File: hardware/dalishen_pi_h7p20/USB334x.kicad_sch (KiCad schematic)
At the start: 21 parts, among them J2 USB_C_Receptacle_USB2.0_16P, J3 USB_A, SW6 SW_DPDT_x2, U20 USB3343, Y1 26M

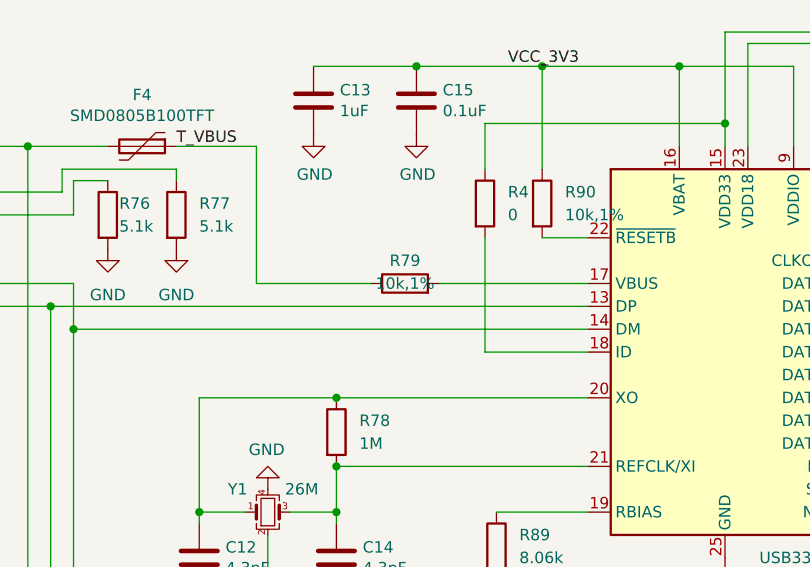
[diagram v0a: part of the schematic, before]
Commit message: [dalishen_pi_h7p20] 待review
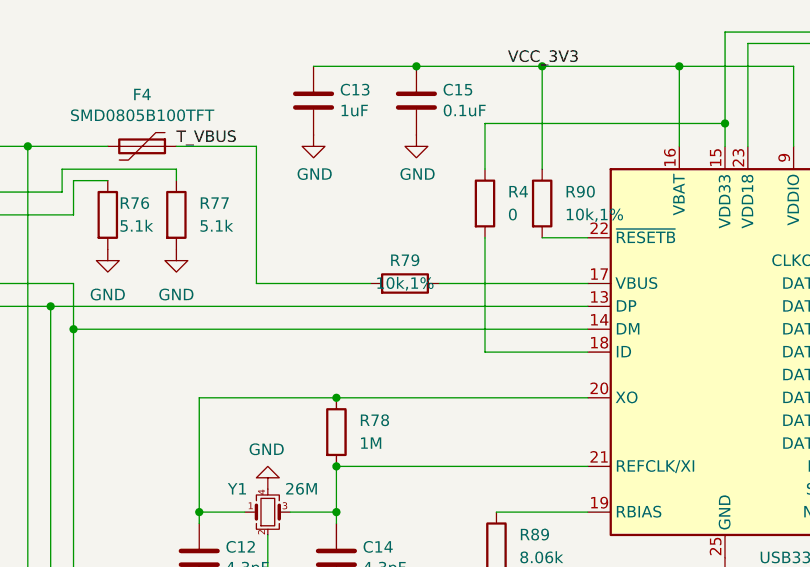
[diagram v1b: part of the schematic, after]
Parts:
- SW6: footprint Button_Switch_SMD:SW_DIP_SPSTx03_Slide_KingTek_DSHP03TJ_W5.25mm_P1.27mm_JPin -> vllogic:SW_PUSH_5.8mm_LOCK_SMT
- U20: footprint Package_DFN_QFN:QFN-24-1EP_4x4mm_P0.5mm_EP2.6x2.6mm -> vllogic:QFN-24-1EP_4x4mm_P0.5mm_EP2.6x2.6mm
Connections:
- net T_VBUS: now also R79.2; no longer R79.1
- net at U20.17 (VBUS): now also R79.1; no longer R79.2
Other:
- moved on the sheet: R79
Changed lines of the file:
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@@
 			)
 		)
-		(property "Footprint" "Button_Switch_SMD:SW_DIP_SPSTx03_Slide_KingTek_DSHP03TJ_W5.25mm_P1.27mm_JPin"
+		(property "Footprint" "vllogic:SW_PUSH_5.8mm_LOCK_SMT"
 			(at 38.1 59.69 0)
 			(effects
@@
 			)
 		)
-		(property "Footprint" "Package_DFN_QFN:QFN-24-1EP_4x4mm_P0.5mm_EP2.6x2.6mm"
+		(property "Footprint" "vllogic:QFN-24-1EP_4x4mm_P0.5mm_EP2.6x2.6mm"
 			(at 210.82 71.12 0)
 			(effects
@@
 	(symbol
 		(lib_id "Device:R")
-		(at 162.56 68.58 90)
+		(at 162.56 68.58 270)
+		(mirror x)
 		(unit 1)
 		(exclude_from_sim no)
@@
 			)
 		)
-		(property "Footprint" "Button_Switch_SMD:SW_DIP_SPSTx03_Slide_KingTek_DSHP03TJ_W5.25mm_P1.27mm_JPin"
+		(property "Footprint" "vllogic:SW_PUSH_5.8mm_LOCK_SMT"
 			(at 38.1 46.99 0)
 			(effects
